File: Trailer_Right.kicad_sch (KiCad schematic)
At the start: 11 parts, among them Q28 IRLZ44N, SW5 SW_SPST, U8 LM339

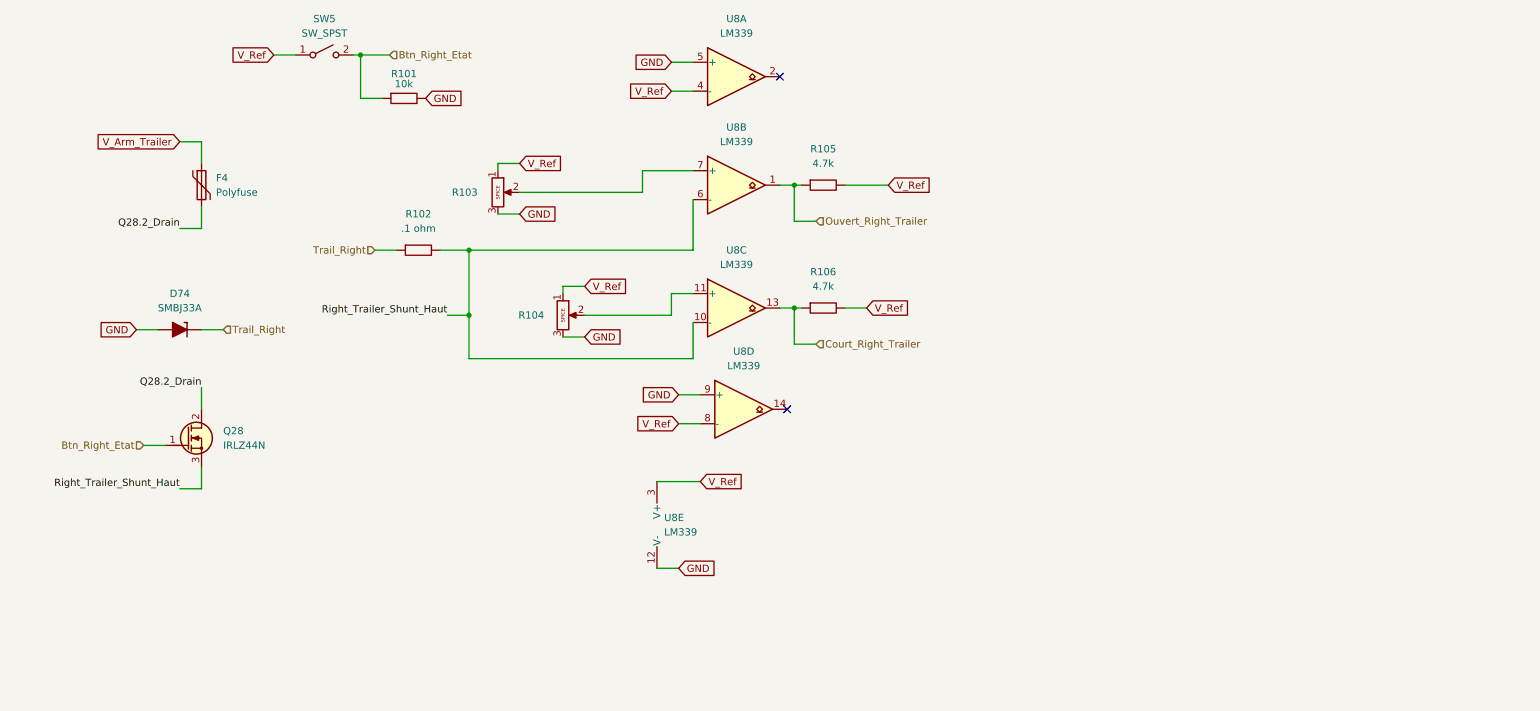
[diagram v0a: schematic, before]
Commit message: Add files via upload
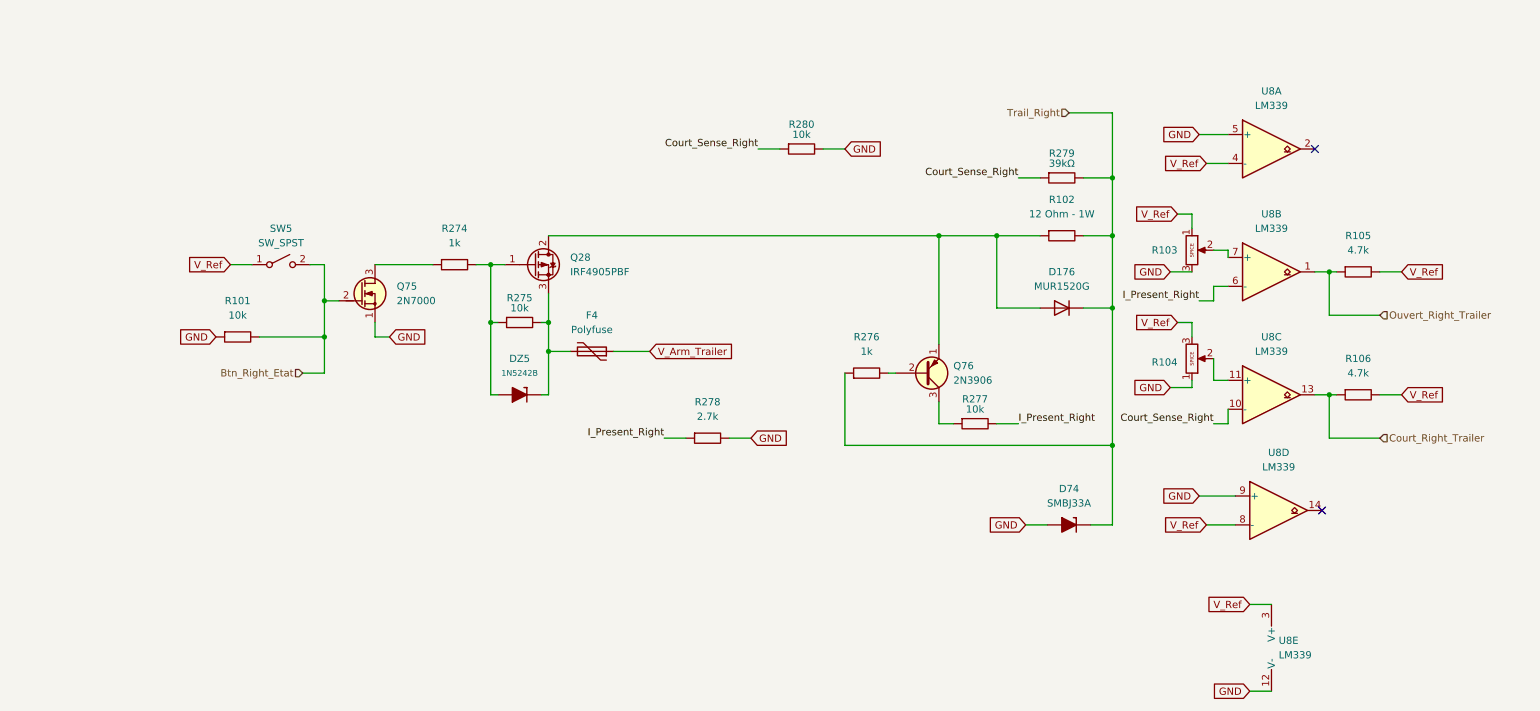
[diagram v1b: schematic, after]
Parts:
- removed Q28: IRLZ44N, PCM_Package_TO_SOT_THT_AKL:TO-220-3_Vertical_GDS, symbol PCM_Transistor_MOSFET_AKL:IRLZ44N
- removed R101: 10k, Resistor_THT:R_Axial_DIN0207_L6.3mm_D2.5mm_P10.16mm_Horizontal, symbol PCM_SL_Resistors:10k
- removed R102: .1 ohm, Resistor_THT:R_Axial_Power_L25.0mm_W9.0mm_P27.94mm, symbol PCM_SL_Resistors:4.7k
- added D176: MUR1520G, Package_TO_SOT_THT:TO-220-2_Vertical, symbol Device:D
- added DZ5: 1N5242B, PCM_Diode_THT_AKL:D_DO-35_SOD27_P7.62mm_Horizontal_Zener, symbol PCM_Diode_Zener_AKL:1N5242B
- added Q28: IRF4905PBF, Package_TO_SOT_THT:TO-220-3_Vertical, symbol Transistor_FET:IRF4905
- added Q75: 2N7000, PCM_Package_TO_SOT_THT_AKL:TO-92_Inline_Wide_SGD, symbol PCM_Transistor_MOSFET_AKL:2N7000
- added Q76: 2N3906, PCM_Package_TO_SOT_THT_AKL:TO-92_Inline_Wide_EBC, symbol PCM_Transistor_BJT_AKL:2N3906
- added R101: 10k, Resistor_THT:R_Axial_DIN0207_L6.3mm_D2.5mm_P10.16mm_Horizontal, symbol PCM_SL_Resistors:4.7k
- added R102: 12 Ohm - 1W, Resistor_THT:R_Axial_DIN0414_L11.9mm_D4.5mm_P15.24mm_Horizontal, symbol PCM_SL_Devices:Resistor_5W
- added R274, R276: 1k, Resistor_THT:R_Axial_DIN0207_L6.3mm_D2.5mm_P10.16mm_Horizontal, symbol PCM_SL_Resistors:1k
- added R275, R277, R280: 10k, Resistor_THT:R_Axial_DIN0207_L6.3mm_D2.5mm_P10.16mm_Horizontal, symbol PCM_SL_Resistors:10k
- added R278: 2.7k, Resistor_THT:R_Axial_DIN0207_L6.3mm_D2.5mm_P10.16mm_Horizontal, symbol PCM_SL_Resistors:2.7k
- added R279: 39kΩ, Resistor_THT:R_Axial_DIN0207_L6.3mm_D2.5mm_P10.16mm_Horizontal, symbol PCM_SL_Resistors:10k
- R103: Etiquette Pot_Right_Ouvert -> (none)
- R104: Etiquette Pot2_Right_Court -> (none)
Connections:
- net Btn_Right_Etat: now also Q75.2 (G), R101.2
- net GND: now also R104.1, Q75.1 (S), R101.1, R278.2, R280.2; no longer R104.3
- net Trail_Right: now also D176.1 (K), R102.2, R276.1, R279.2
- net V_Ref: now also R104.3; no longer R104.1
- net Q28.2_Drain: no longer names the net of F4.2
- net Q28.2_Drain: now also DZ5.1 (K), Q28.3 (S), R275.2
- net Right_Trailer_Shunt_Haut renamed Court_Sense_Right
- net Court_Sense_Right: now also R279.1, R280.1; no longer U8.6 (-)
- new net: D176.2 (A), Q28.2 (D), Q76.1 (E), R102.1
- new net: Q76.2 (B), R276.2
- new net: Q76.3 (C), R277.1
- new net: Q75.3 (D), R274.1
- new net: DZ5.2 (A), Q28.1 (G), R274.2, R275.1
- new net I_Present_Right: R277.2, R278.1, U8.6 (-)
